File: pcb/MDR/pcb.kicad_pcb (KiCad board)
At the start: 2 copper layers, 40.1 x 52 mm, 13 parts, among them J1 1x3f Tmp Sens, J2 1x4f Screen, J3 1x8f Digital Pin Headers, J4 1x2f LED, J5 1x3f tmp switch, J6 1x2F 5V in, U1 ATmega328-P, Y1 16MHz

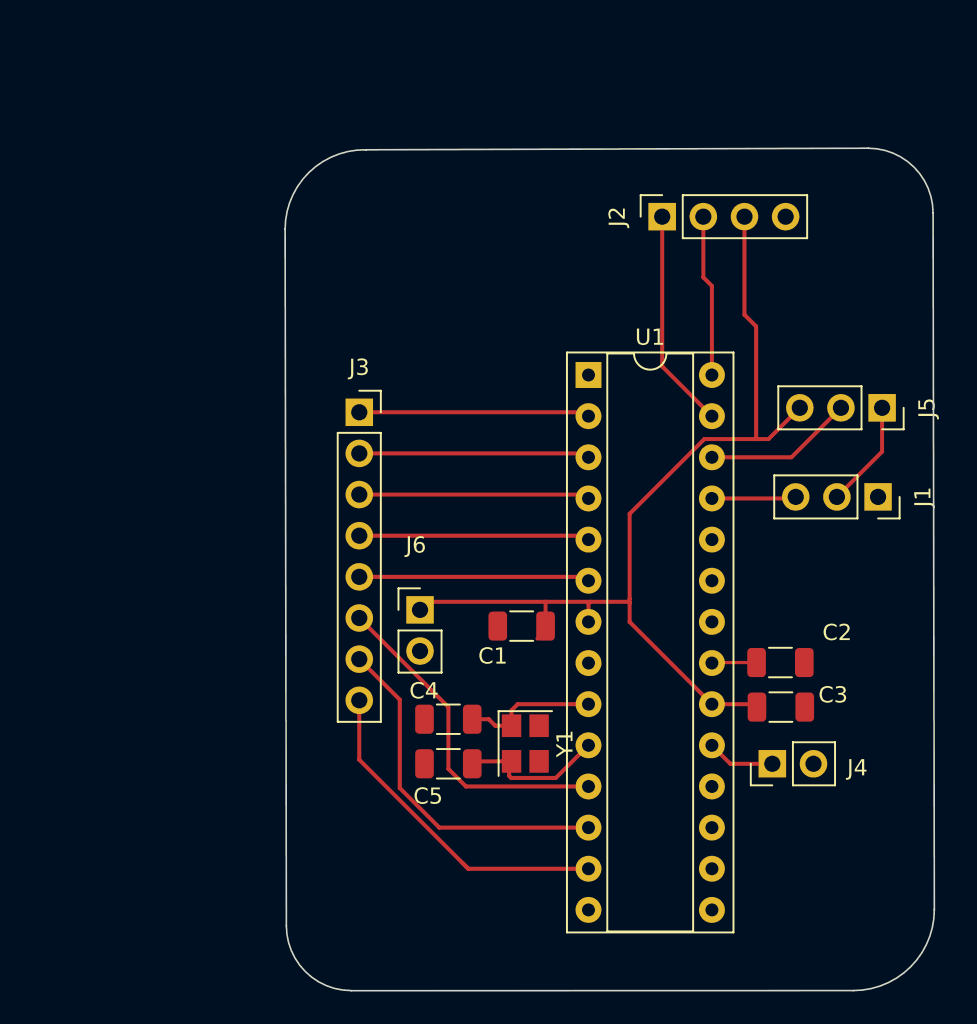
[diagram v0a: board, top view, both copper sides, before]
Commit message: cdr pcb
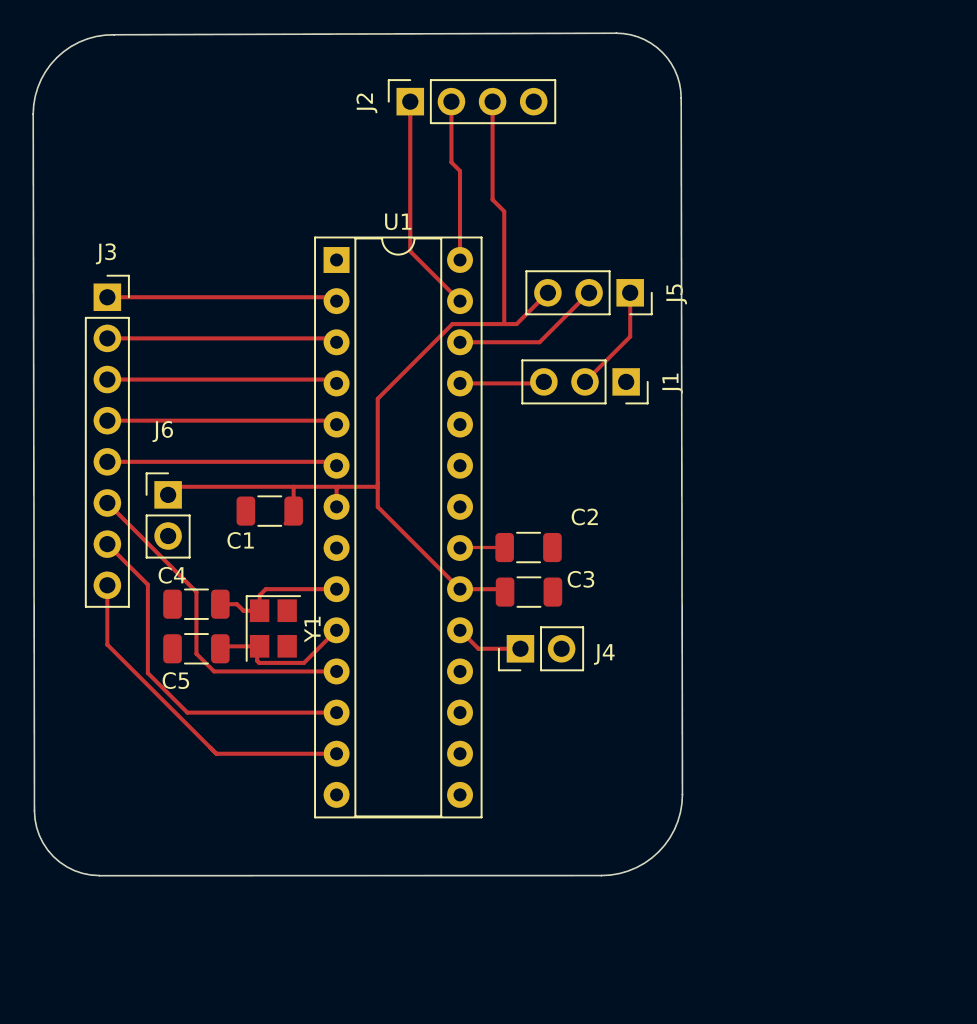
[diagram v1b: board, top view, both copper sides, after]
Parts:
- moved J1 17.1 mm to (125.5, 80.7)
- moved J5 17.1 mm to (125.7, 75.2)
- moved C1 17.1 mm to (103.5, 88.7)
- moved C3 17.1 mm to (119.5, 93.7)
- moved U1 17.1 mm to (107.6, 73.2)
- moved C2 17.1 mm to (119.5, 90.9)
- moved C4 17.1 mm to (99.0, 94.4)
- moved C5 17.1 mm to (99.0, 97.2)
- moved J2 17.1 mm to (112.2, 63.4)
- moved J3 17.1 mm to (93.5, 75.5)
- moved J4 17.1 mm to (119.0, 97.2)
- moved J6 17.1 mm to (97.2, 87.7)
- moved Y1 17.1 mm to (103.7, 95.9)
